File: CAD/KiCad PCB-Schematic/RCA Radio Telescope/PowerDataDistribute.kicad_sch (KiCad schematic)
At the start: 13 parts, among them J7 USB_A, J8 USB_A, Q1 DMP2008UFG-7, U13 MIC23050-SYML-TR

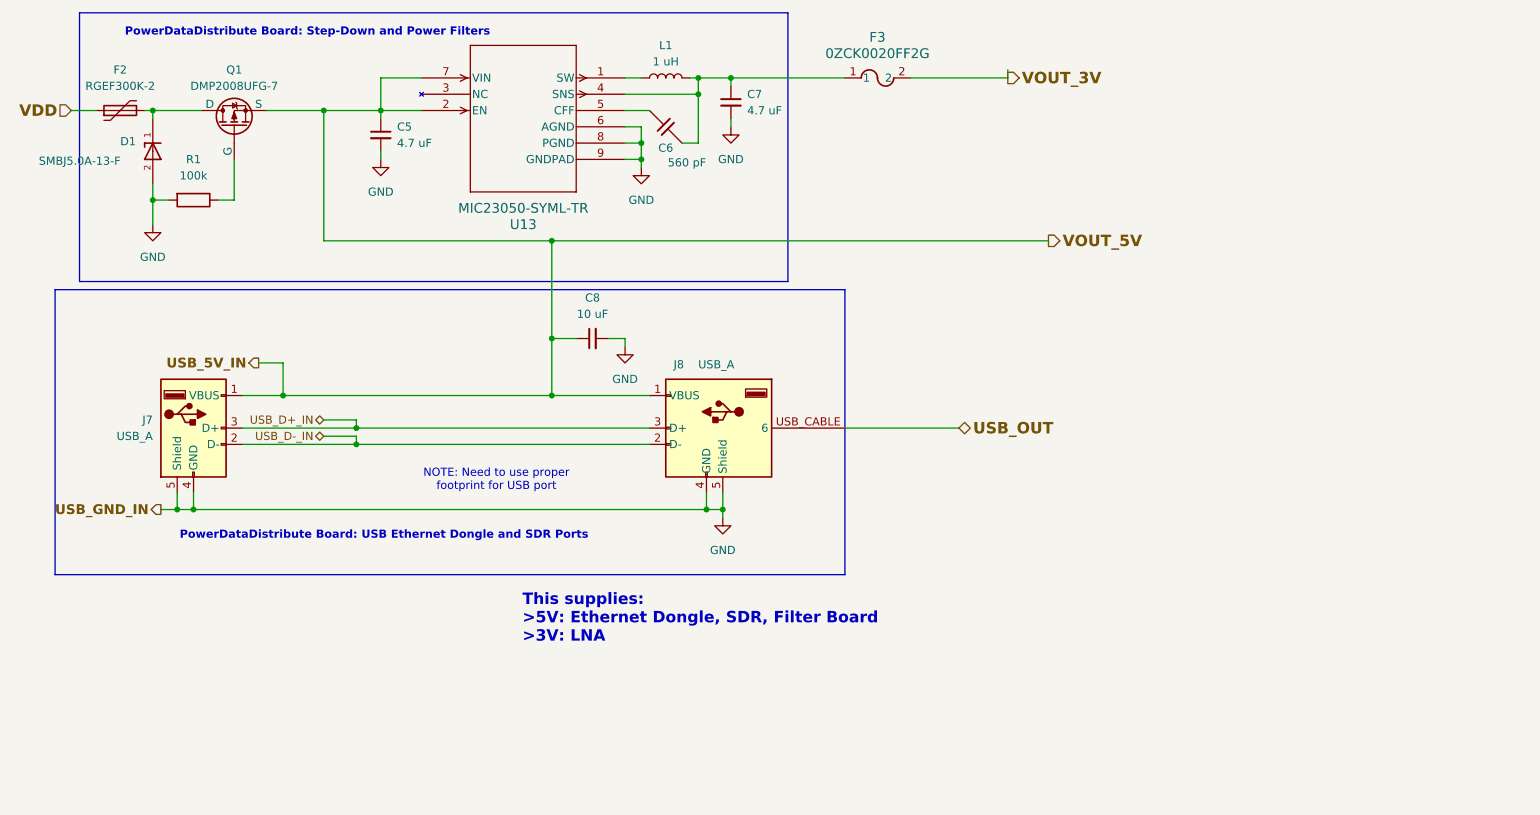
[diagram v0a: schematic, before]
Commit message: V1.5 Schematic and 1.4 PCB Layout
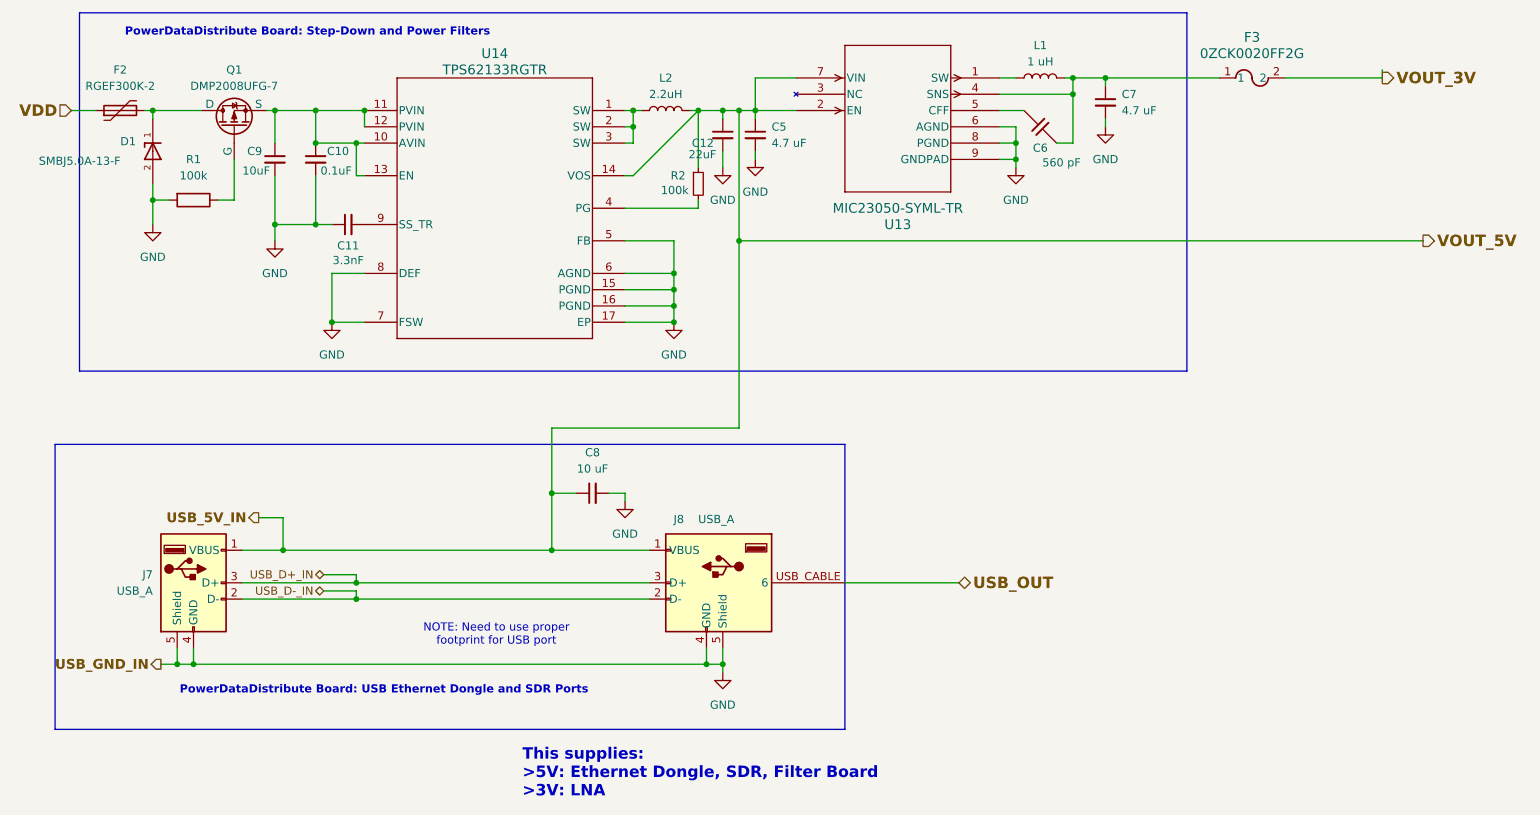
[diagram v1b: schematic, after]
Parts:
- added C10: 0.1uF, Capacitor_SMD:C_0805_2012Metric, symbol Device:C_Small
- added C11: 3.3nF, Capacitor_SMD:C_0805_2012Metric, symbol Device:C_Small
- added C12: 22uF, Capacitor_SMD:C_0805_2012Metric, symbol Device:C_Small
- added C9: 10uF, Capacitor_SMD:C_0805_2012Metric, symbol Device:C_Small
- added L2: 2.2uH, Inductor_SMD:L_0805_2012Metric, symbol Device:L
- added R2: 100k, Resistor_SMD:R_0805_2012Metric, symbol Device:R_Small
- added U14: TPS62133RGTR, TPS62133RGTR:RGT0016C, symbol TPS62133RGTR:TPS62133RGTR
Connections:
- net GND: now also C10.2, C11.1, C12.2, C9.2, U14.15 (PGND), U14.16 (PGND), U14.17 (EP), U14.5 (FB), U14.6 (AGND), U14.7 (FSW), U14.8 (DEF)
- net USB_5V_IN: now also C12.1, L2.2, R2.1, U14.14 (VOS); no longer Q1.3 (S)
- new net: L2.1, U14.1 (SW), U14.2 (SW), U14.3 (SW)
- new net: C10.1, C9.1, Q1.3 (S), U14.10 (AVIN), U14.11 (PVIN), U14.12 (PVIN), U14.13 (EN)
- new net: R2.2, U14.4 (PG)
- new net: C11.2, U14.9 (SS_TR)
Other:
- moved on the sheet: C5, C6, C7, C8, F3, J7, J8, L1, U13
